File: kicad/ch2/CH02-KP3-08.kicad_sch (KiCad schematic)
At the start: 5 parts

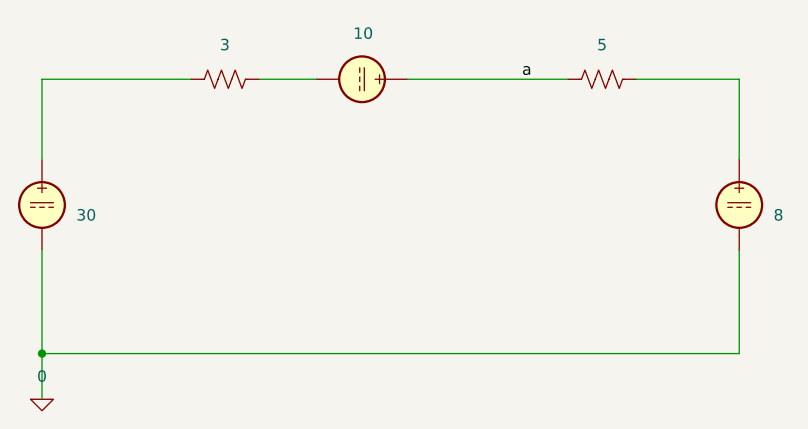
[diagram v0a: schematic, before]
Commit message: regular
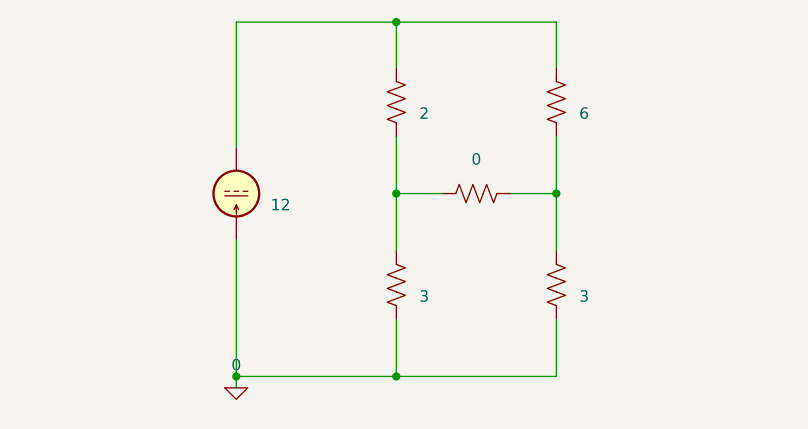
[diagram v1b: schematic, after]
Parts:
- removed R4: 3, symbol Device:R_US
- removed R5: 5, symbol Device:R_US
- removed V3: 30, symbol Simulation_SPICE:VDC
- removed V4: 10, symbol Simulation_SPICE:VDC
- removed V5: 8, symbol Simulation_SPICE:VDC
- added I5: 12, symbol Simulation_SPICE:IDC
- added R24: 2, symbol Device:R_US
- added R25: 6, symbol Device:R_US
- added R26, R27: 3, symbol Device:R_US
- added R28: 0, symbol Device:R_US
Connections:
- net 0: now also I5.1, R26.2, R27.2
- new net: R25.2, R27.1, R28.1
- new net: I5.2, R24.1, R25.1
- new net: R24.2, R26.1, R28.2
